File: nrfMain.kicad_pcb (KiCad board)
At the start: 4 copper layers, 40.2 x 68.8 mm, 76 parts, among them J1 FTSH-105-01-F-DV-P-TR, J2 USB_C_Receptacle, J3 Conn_01x03, J4 Conn_01x04, J5 2337019-1, M1 Motor_Servo, M2 Motor_Servo, M3 Motor_Servo, M4 Motor_Servo, M5 Motor_Servo, M6 Motor_Servo, Q1 Q_NMOS_GSD, Q2 Q_NMOS_GSD, Q3 DMG2301L, SW1 SW_Push, U1 nRF52840, U3 MCP73831-2-OT, U4 MAX17048, U5 MX25R6435FZAIL0, U6 AP22814AW5, U8 LD39150DT33, Y1 32MHz, Y2 32.768kHz

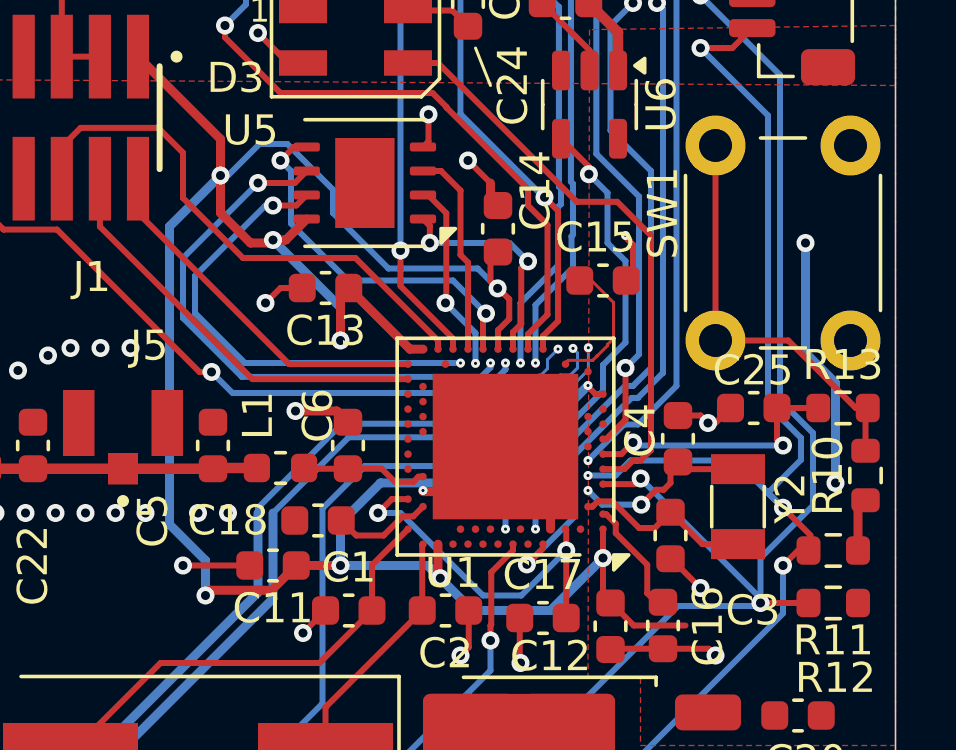
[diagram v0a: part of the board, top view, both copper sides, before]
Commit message: Made modifications from fabrication
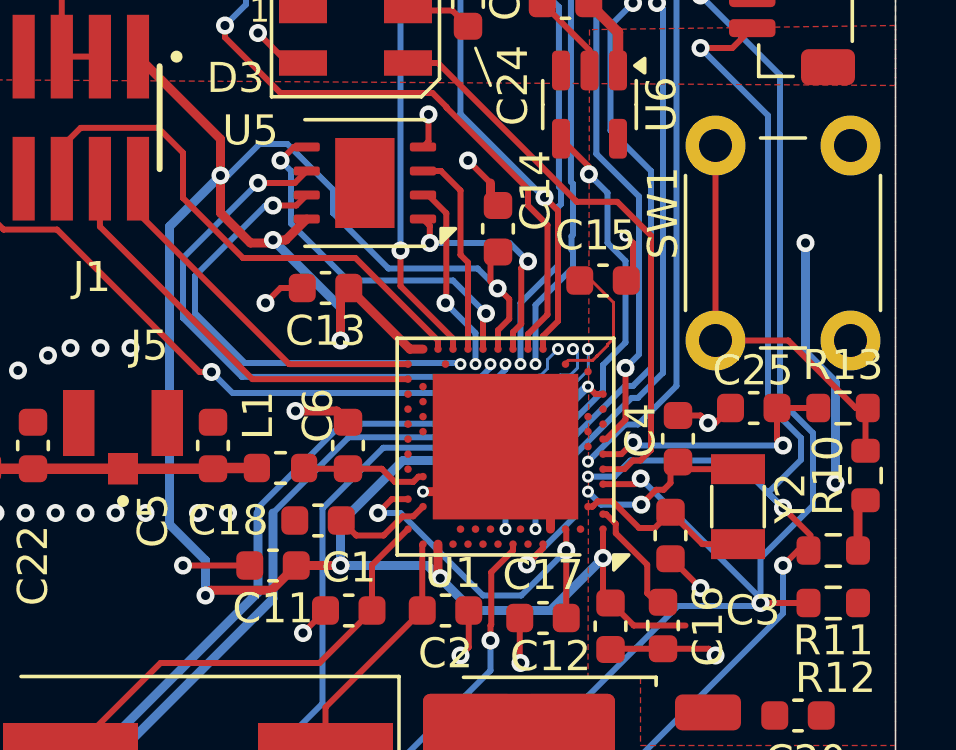
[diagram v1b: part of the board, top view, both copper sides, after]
